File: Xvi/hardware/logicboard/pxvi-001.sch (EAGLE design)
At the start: 68 parts, among them J1 MKR, J5 SPI, J7 DIN5, K1 G5V1, Q1 60V/32A/35mΩ, Q10 60V/32A/35mΩ, Q11 60V/32A/35mΩ, Q12 60V/32A/35mΩ, Q13 60V/32A/35mΩ, Q14 60V/32A/35mΩ, Q15 60V/32A/35mΩ, Q16 60V/32A/35mΩ, Q2 60V/32A/35mΩ, Q3 60V/32A/35mΩ, Q4 60V/32A/35mΩ, Q5 60V/32A/35mΩ, Q6 60V/32A/35mΩ, Q7 60V/32A/35mΩ, Q8 60V/32A/35mΩ, Q9 60V/32A/35mΩ, T1 2SC1815, U1 DS18B20, X1 ADAFRUIT-PCA9685, X2 MKDSN1,5/2-5,08

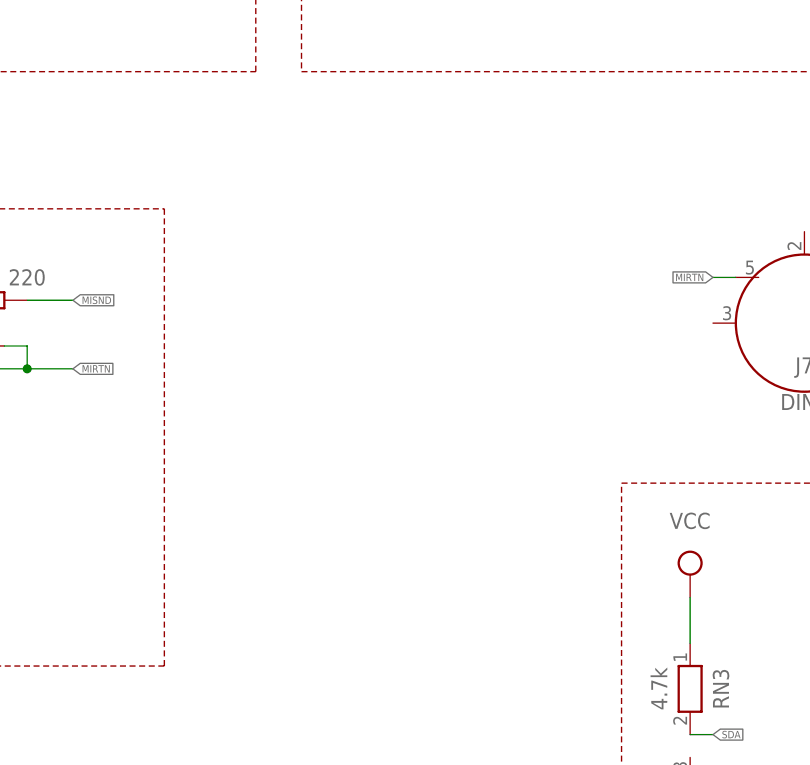
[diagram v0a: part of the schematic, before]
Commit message: Qwiic con.
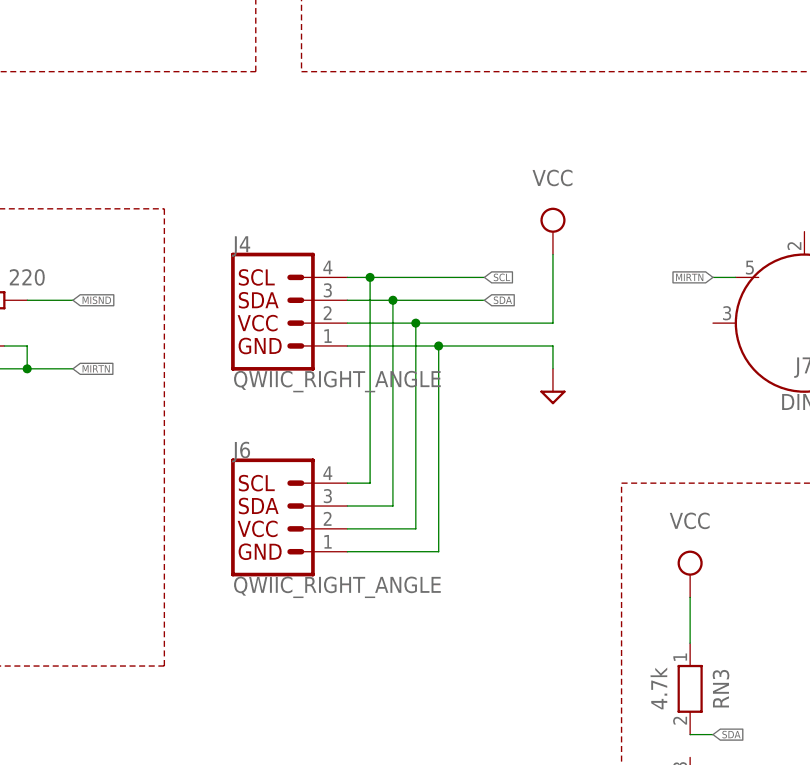
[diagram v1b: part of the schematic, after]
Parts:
- added J4, J6: QWIIC_RIGHT_ANGLE, SparkFun-Connectors:QWIIC_CONNECTORJS-1MM
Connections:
- net GND: now also J4.1, J6.1
- net SCL: now also J4.4, J6.4
- net SDA: now also J4.3, J6.3
- net VCC: now also J4.2, J6.2
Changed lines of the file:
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@@
 <layer number="56" name="wert" color="7" fill="1" visible="no" active="no"/>
 <layer number="57" name="tCAD" color="7" fill="1" visible="no" active="no"/>
+<layer number="58" name="bCAD" color="7" fill="1" visible="no" active="no"/>
 <layer number="59" name="tCarbon" color="7" fill="1" visible="no" active="no"/>
 <layer number="60" name="bCarbon" color="7" fill="1" visible="no" active="no"/>
@@
 <layer number="128" name="_bValues" color="7" fill="1" visible="yes" active="yes"/>
 <layer number="129" name="Mask" color="7" fill="1" visible="yes" active="yes"/>
+<layer number="130" name="SMDSTROOK" color="7" fill="1" visible="no" active="no"/>
 <layer number="131" name="tAdjust" color="7" fill="1" visible="no" active="yes"/>
 <layer number="132" name="bAdjust" color="7" fill="1" visible="no" active="yes"/>
+<layer number="133" name="bottom_silk" color="7" fill="1" visible="no" active="no"/>
+<layer number="134" name="silk_top" color="7" fill="1" visible="no" active="no"/>
+<layer number="135" name="silk_bottom" color="7" fill="1" visible="no" active="no"/>
+<layer number="136" name="silktop" color="7" fill="1" visible="no" active="no"/>
+<layer number="137" name="silkbottom" color="7" fill="1" visible="no" active="no"/>
+<layer number="138" name="EEE" color="7" fill="1" visible="no" active="no"/>
+<layer number="139" name="_tKeepout" color="7" fill="1" visible="no" active="no"/>
+<layer number="140" name="mbKeepout" color="7" fill="1" visible="no" active="no"/>
+<layer number="141" name="ASSEMBLY_TOP" color="7" fill="1" visible="no" active="no"/>
+<layer number="142" name="mbRestrict" color="7" fill="1" visible="no" active="no"/>
+<layer number="143" name="PLACE_BOUND_TOP" color="7" fill="1" visible="no" active="no"/>
 <layer number="144" name="Drill_legend" color="7" fill="1" visible="yes" active="yes"/>
+<layer number="145" name="DrillLegend_01-16" color="7" fill="1" visible="no" active="no"/>
+<layer number="146" name="DrillLegend_01-20" color="7" fill="1" visible="no" active="no"/>
+<layer number="147" name="PIN_NUMBER" color="7" fill="1" visible="no" active="no"/>
+<layer number="148" name="DrillLegend_01-20" color="7" fill="1" visible="no" active="no"/>
+<layer number="149" name="DrillLegend_02-15" color="7" fill="1" visible="no" active="no"/>
 <layer number="150" name="Notes" color="7" fill="1" visible="no" active="yes"/>
 <layer number="151" name="HeatSink" color="7" fill="1" visible="yes" active="yes"/>
@@
 <layer number="154" name="FabDoc2" color="2" fill="1" visible="no" active="no"/>
 <layer number="155" name="FabDoc3" color="7" fill="15" visible="no" active="no"/>
+<layer number="156" name="gesam-Maß" color="7" fill="1" visible="no" active="no"/>
+<layer number="157" name="FaceMchng" color="7" fill="1" visible="no" active="no"/>
+<layer number="158" name="FaceMMeas" color="7" fill="1" visible="no" active="no"/>
+<layer number="159" name="Geh-Bear2" color="7" fill="1" visible="no" active="no"/>
+<layer number="160" name="Topologie" color="7" fill="1" visible="no" active="no"/>
+<layer number="161" name="tomplace2" color="7" fill="1" visible="no" active="no"/>
+<layer number="166" name="AntennaArea" color="7" fill="1" visible="no" active="no"/>
+<layer number="168" name="4mmHeightArea" color="7" fill="1" visible="no" active="no"/>
+<layer number="191" name="mNets" color="7" fill="1" visible="no" active="no"/>
+<layer number="192" name="mBusses" color="7" fill="1" visible="no" active="no"/>
+<layer number="193" name="mPins" color="7" fill="1" visible="no" active="no"/>
+<layer number="194" name="mSymbols" color="7" fill="1" visible="no" active="no"/>
+<layer number="195" name="mNames" color="7" fill="1" visible="no" active="no"/>
+<layer number="196" name="mValues" color="7" fill="1" visible="no" active="no"/>
 <layer number="199" name="Contour" color="7" fill="1" visible="yes" active="yes"/>
 <layer number="200" name="200bmp" color="1" fill="10" visible="yes" active="yes"/>
@@
 <layer number="250" name="Descript" color="7" fill="1" visible="no" active="no"/>
 <layer number="251" name="SMDround" color="7" fill="1" visible="no" active="no"/>
+<layer number="252" name="BR-BS" color="7" fill="1" visible="no" active="no"/>
+<layer number="253" name="Extra" color="7" fill="1" visible="no" active="no"/>
 <layer number="254" name="cooling" color="7" fill="1" visible="yes" active="yes"/>
 <layer number="255" name="routoute" color="7" fill="1" visible="yes" active="yes"/>
@@
 <part name="SUPPLY38" library="supply2" library_urn="urn:adsk.eagle:library:372" deviceset="VCC" device=""/>
 <part name="SUPPLY39" library="supply2" deviceset="GND" device=""/>
+<part name="J4" library="SparkFun-Connectors" library_urn="urn:adsk.eagle:library:513" deviceset="QWIIC_CONNECTOR" device="JS-1MM" package3d_urn="urn:adsk.eagle:package:41390393/1" value="QWIIC_RIGHT_ANGLE"/>
+<part name="J6" library="SparkFun-Connectors" library_urn="urn:adsk.eagle:library:513" deviceset="QWIIC_CONNECTOR" device="JS-1MM" package3d_urn="urn:adsk.eagle:package:41390393/1" value="QWIIC_RIGHT_ANGLE"/>
+<part name="SUPPLY40" library="supply2" library_urn="urn:adsk.eagle:library:372" deviceset="VCC" device=""/>
+<part name="SUPPLY41" library="supply2" deviceset="GND" device=""/>
 </parts>
 <sheets>
@@
 </instance>
 <instance part="SUPPLY39" gate="GND" x="350.52" y="129.54" smashed="yes"/>
+<instance part="J4" gate="J1" x="215.9" y="139.7" smashed="yes">
+<attribute name="VALUE" x="210.82" y="134.366" size="1.778" layer="96" font="vector" align="top-left"/>
+<attribute name="NAME" x="210.82" y="147.574" size="1.778" layer="95" font="vector"/>
+</instance>
+<instance part="J6" gate="J1" x="215.9" y="116.84" smashed="yes">
+<attribute name="VALUE" x="210.82" y="111.506" size="1.778" layer="96" font="vector" align="top-left"/>
+<attribute name="NAME" x="210.82" y="124.714" size="1.778" layer="95" font="vector"/>
+</instance>
+<instance part="SUPPLY40" gate="G$1" x="246.38" y="149.86" smashed="yes">
+<attribute name="VALUE" x="246.38" y="154.94" size="1.778" layer="96" align="bottom-center"/>
+</instance>
+<instance part="SUPPLY41" gate="GND" x="246.38" y="132.08" smashed="yes"/>
 </instances>
 <busses>
@@
 <wire x1="350.52" y1="147.32" x2="350.52" y2="132.08" width="0.1524" layer="91"/>
 </segment>
+<segment>
+<pinref part="J4" gate="J1" pin="1"/>
+<wire x1="223.52" y1="137.16" x2="233.68" y2="137.16" width="0.1524" layer="91"/>
+<wire x1="233.68" y1="137.16" x2="246.38" y2="137.16" width="0.1524" layer="91"/>
+<wire x1="246.38" y1="137.16" x2="246.38" y2="134.62" width="0.1524" layer="91"/>
+<pinref part="J6" gate="J1" pin="1"/>
+<wire x1="223.52" y1="114.3" x2="233.68" y2="114.3" width="0.1524" layer="91"/>
+<wire x1="233.68" y1="114.3" x2="233.68" y2="137.16" width="0.1524" layer="91"/>
+<junction x="233.68" y="137.16"/>
+<pinref part="SUPPLY41" gate="GND" pin="GND"/>
+</segment>
 </net>
 <net name="VCC" class="2">
@@
 <junction x="358.14" y="157.48"/>
 </segment>
+<segment>
+<pinref part="J4" gate="J1" pin="2"/>
+<wire x1="223.52" y1="139.7" x2="231.14" y2="139.7" width="0.1524" layer="91"/>
+<pinref part="J6" gate="J1" pin="2"/>
+<wire x1="223.52" y1="116.84" x2="231.14" y2="116.84" width="0.1524" layer="91"/>
+<wire x1="231.14" y1="116.84" x2="231.14" y2="139.7" width="0.1524" layer="91"/>
+<junction x="231.14" y="139.7"/>
+<wire x1="231.14" y1="139.7" x2="246.38" y2="139.7" width="0.1524" layer="91"/>
+<wire x1="246.38" y1="139.7" x2="246.38" y2="147.32" width="0.1524" layer="91"/>
+<pinref part="SUPPLY40" gate="G$1" pin="VCC"/>
+</segment>
 </net>
 <net name="RST" class="0">
@@
 <label x="88.9" y="63.5" size="0.8128" layer="95" xref="yes"/>
 </segment>
+<segment>
+<pinref part="J4" gate="J1" pin="3"/>
+<wire x1="223.52" y1="142.24" x2="228.6" y2="142.24" width="0.1524" layer="91"/>
+<pinref part="J6" gate="J1" pin="3"/>
+<wire x1="228.6" y1="142.24" x2="238.76" y2="142.24" width="0.1524" layer="91"/>
+<wire x1="228.6" y1="142.24" x2="228.6" y2="119.38" width="0.1524" layer="91"/>
+<wire x1="228.6" y1="119.38" x2="223.52" y2="119.38" width="0.1524" layer="91"/>
+<junction x="228.6" y="142.24"/>
+<label x="238.76" y="142.24" size="0.8128" layer="95" xref="yes"/>
+</segment>
 </net>
 <net name="SCL" class="0">
@@
 <label x="88.9" y="60.96" size="0.8128" layer="95" xref="yes"/>
 </segment>
+<segment>
+<pinref part="J4" gate="J1" pin="4"/>
+<wire x1="223.52" y1="144.78" x2="226.06" y2="144.78" width="0.1524" layer="91"/>
+<pinref part="J6" gate="J1" pin="4"/>
+<wire x1="226.06" y1="144.78" x2="238.76" y2="144.78" width="0.1524" layer="91"/>
+<wire x1="223.52" y1="121.92" x2="226.06" y2="121.92" width="0.1524" layer="91"/>
+<wire x1="226.06" y1="121.92" x2="226.06" y2="144.78" width="0.1524" layer="91"/>
+<junction x="226.06" y="144.78"/>
+<label x="238.76" y="144.78" size="0.8128" layer="95" xref="yes"/>
+</segment>
 </net>
